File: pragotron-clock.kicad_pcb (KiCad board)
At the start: 2 copper layers, 2 parts, among them U1 L293D, U2 ESP32_DEVCITV1

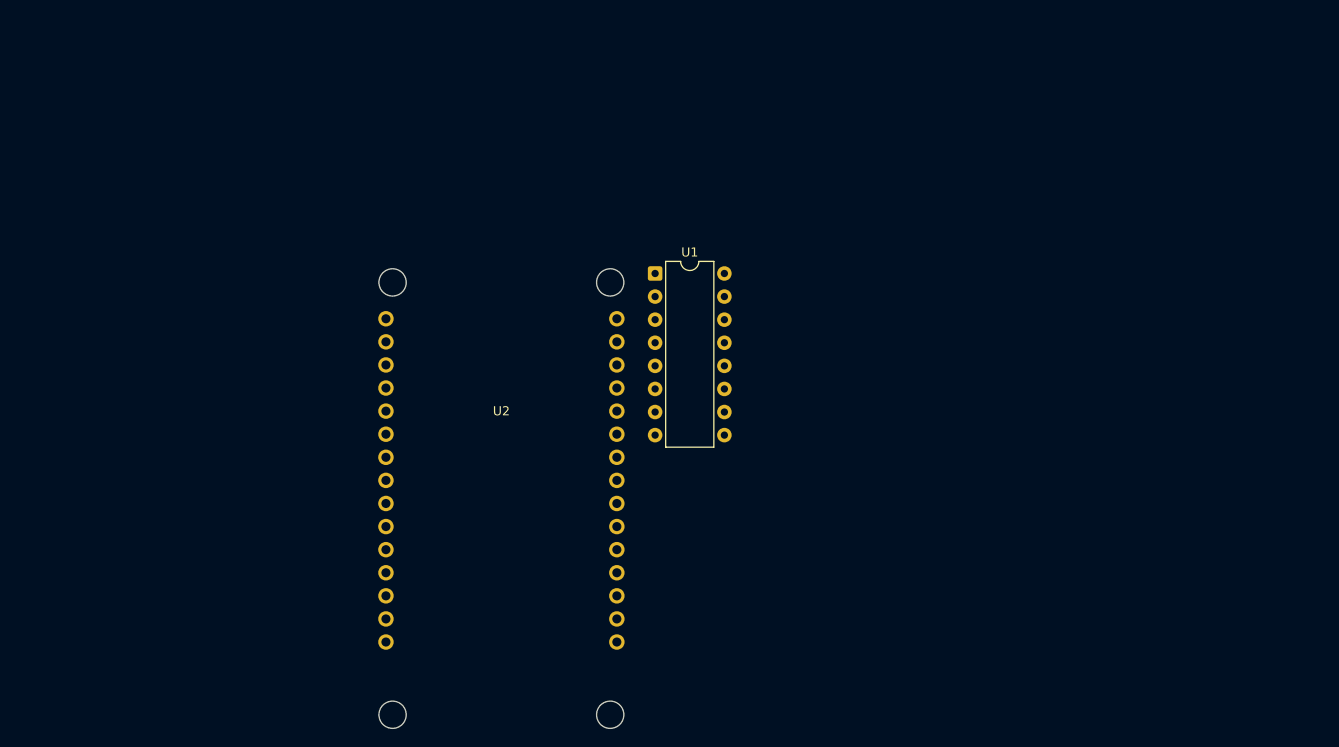
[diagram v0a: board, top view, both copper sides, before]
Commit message: control schematic
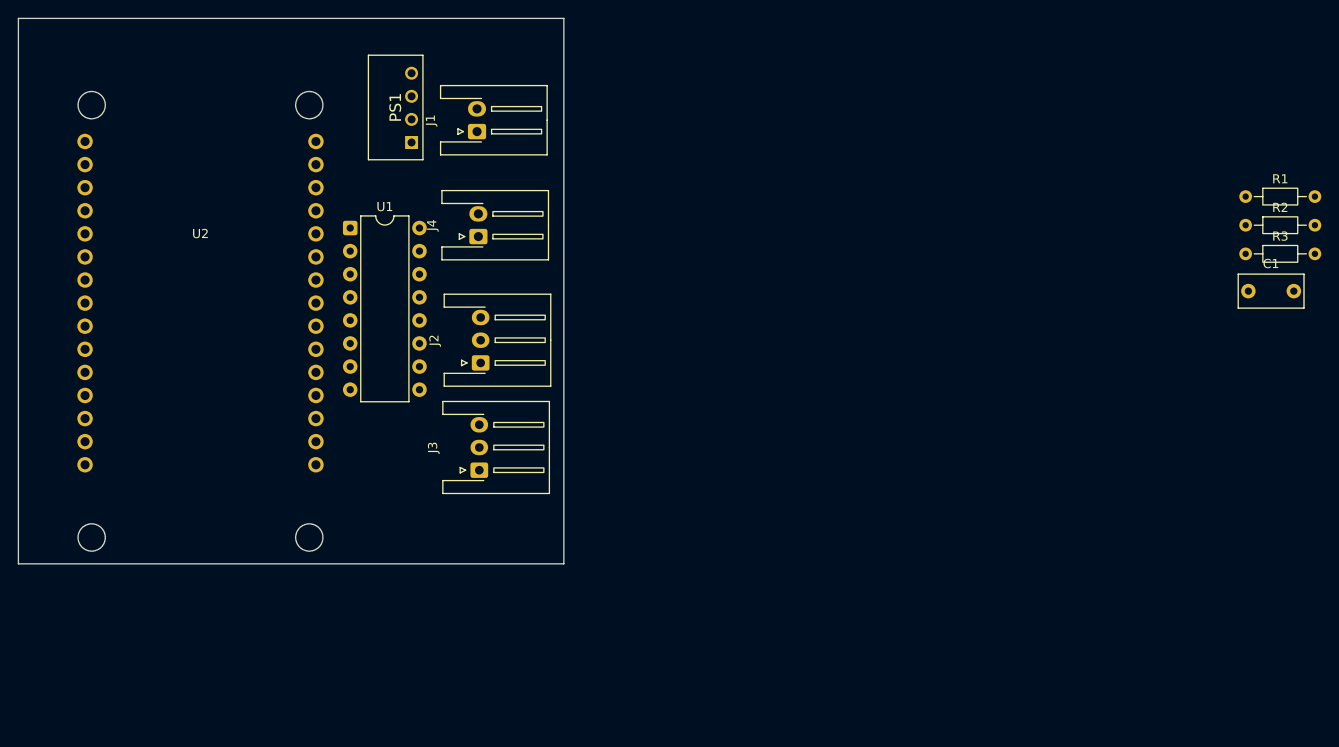
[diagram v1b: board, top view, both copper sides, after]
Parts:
- added C1: 10u 100V MLCC, Capacitor_THT:C_Rect_L7.0mm_W3.5mm_P5.00mm, F.Cu at (215.3, 80.0)
- added J1: Conn_01x02, Connector_JST:JST_XH_S2B-XH-A-1_1x02_P2.50mm_Horizontal, F.Cu at (130.4, 62.5)
- added J2: Conn_01x03, Connector_JST:JST_XH_S3B-XH-A-1_1x03_P2.50mm_Horizontal, F.Cu at (130.8, 87.9)
- added J3: Conn_01x03, Connector_JST:JST_XH_S3B-XH-A-1_1x03_P2.50mm_Horizontal, F.Cu at (130.7, 99.7)
- added J4: Conn_01x02, Connector_JST:JST_XH_S2B-XH-A-1_1x02_P2.50mm_Horizontal, F.Cu at (130.6, 74.0)
- added PS1: ROE-2405S, JS_Local:ROE1205S, F.Cu at (123.2, 63.6)
- added R1: 47K, Resistor_THT:R_Axial_DIN0204_L3.6mm_D1.6mm_P7.62mm_Horizontal, F.Cu at (215.0, 69.6)
- added R2: 10K, Resistor_THT:R_Axial_DIN0204_L3.6mm_D1.6mm_P7.62mm_Horizontal, F.Cu at (215.0, 72.8)
- added R3: 10K, Resistor_THT:R_Axial_DIN0204_L3.6mm_D1.6mm_P7.62mm_Horizontal, F.Cu at (215.0, 75.9)
- moved U2 38.4 mm to (87.3, 63.5)
- moved U1 33.9 mm to (116.5, 73.1)
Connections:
- U1 pad 12: unconnected-(U1-GND-Pad12) -> GND
- U1 pad 13: unconnected-(U1-GND-Pad13) -> GND
- U1 pad 16: +5V -> Net-(J2-Pin_1)
- U1 pad 4: unconnected-(U1-GND-Pad4) -> GND
- U1 pad 5: unconnected-(U1-GND-Pad5) -> GND
- U1 pad 9: unconnected-(U1-EN3,4-Pad9) -> GND
- U2 pad 15: unconnected-(U2-VIN-Pad15) -> +5V
- U2 pad 30: unconnected-(U2-3V3-Pad30) -> Net-(J2-Pin_1)
- U2 pad 5: unconnected-(U2-D35-Pad5) -> Net-(J2-Pin_3)
- U2 pad 6: unconnected-(U2-D32-Pad6) -> Net-(J3-Pin_3)
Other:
- board outline added: 60 x 60 mm
